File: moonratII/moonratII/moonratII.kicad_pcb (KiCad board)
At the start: 2 copper layers, 97.4 x 65.6 mm, 24 parts, among them J1 Barrel_Jack_Switch_SMT, J3 Conn_02x05_Odd_Even, J4 Screw_Terminal_01x06, J5 Screw_Terminal_01x06, J6 Conn_02x05_Odd_Even, J7 Screw_Terminal_01x02, Q1 IRF520N, Q2 BSS138, SW1 6mm 2 Pin Tact NO Breadboard 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, SW2 6mm 2 Pin Tact NO Breadboard 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, SW3 6mm 2 Pin Tact NO Breadboard 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, U1 TMP36xS

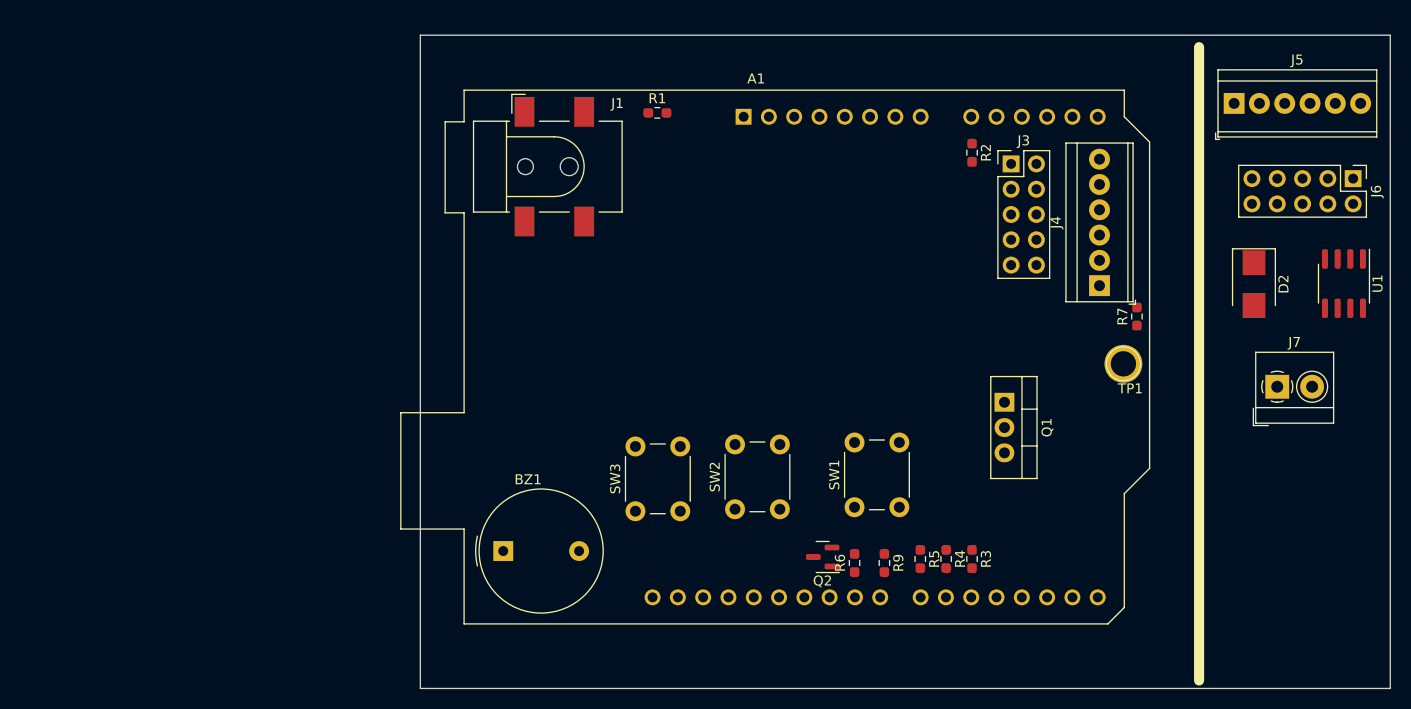
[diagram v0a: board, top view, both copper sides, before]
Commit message: Add more PCB 3D models. Place and lock down mounting holes.
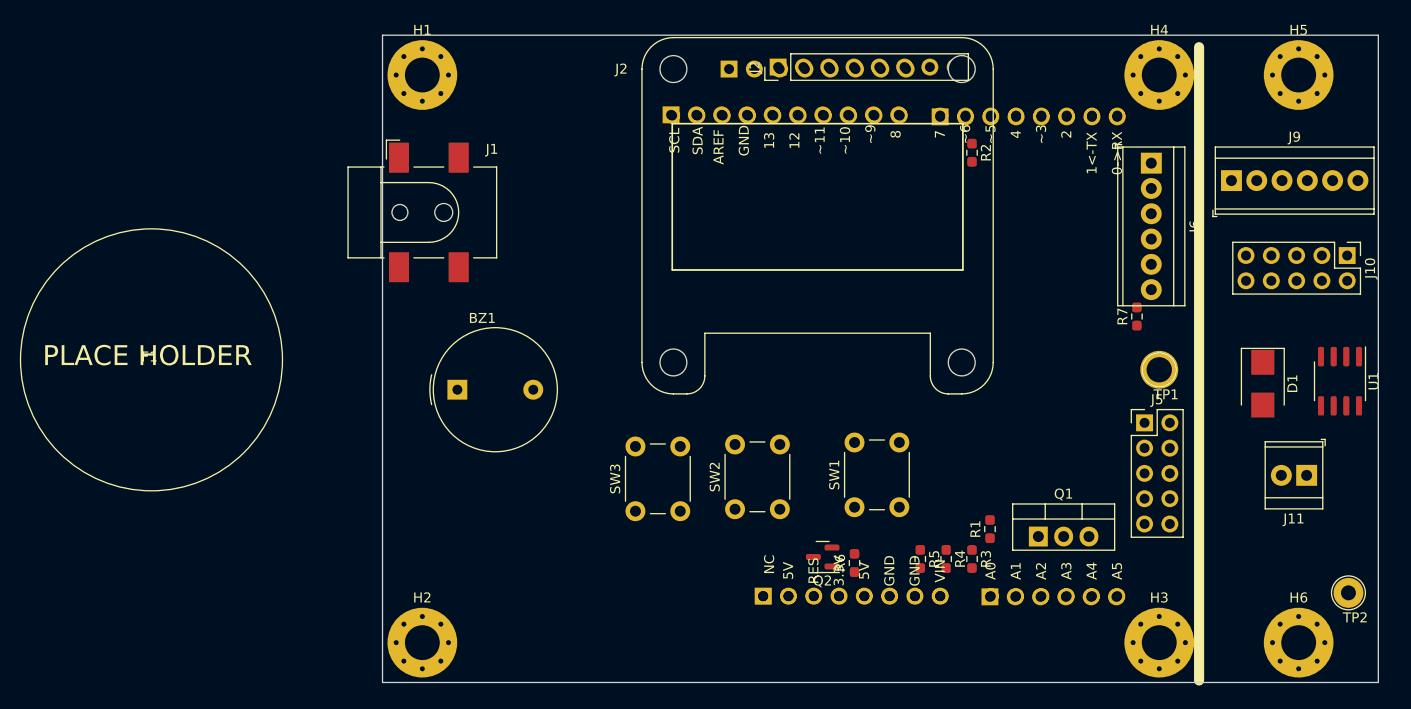
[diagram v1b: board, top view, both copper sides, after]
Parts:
- removed D2: Schottky 2A, Diode_SMD:D_SMB
- removed R9: 1K, Resistor_SMD:R_0603_1608Metric_Pad0.98x0.95mm_HandSolder
- added D1: Schottky 2A, Diode_SMD:D_SMB, F.Cu at (188.4, 95.0)
- added F1: Polyfuse 6A, GeneralPurposeAlarmDevicePCB:PlaceHolderOpossum, F.Cu at (76.6, 92.8)
- added H1: MountingHole_Pad_3.5mm, GeneralPurposeAlarmDevicePCB:MountingHole_3.5mm_Pad_Via, F.Cu at (104.0, 64.0)
- added H2: MountingHole_Pad_3.5mm, GeneralPurposeAlarmDevicePCB:MountingHole_3.5mm_Pad_Via, F.Cu at (104.0, 121.0)
- added H3: MountingHole_Pad_3.5mm, GeneralPurposeAlarmDevicePCB:MountingHole_3.5mm_Pad_Via, F.Cu at (178.0, 121.0)
- added H4: MountingHole_Pad_3.5mm, GeneralPurposeAlarmDevicePCB:MountingHole_3.5mm_Pad_Via, F.Cu at (178.0, 64.0)
- added H5: MountingHole_Pad_3.5mm, GeneralPurposeAlarmDevicePCB:MountingHole_3.5mm_Pad_Via, F.Cu at (192.0, 64.0)
- added H6: MountingHole_Pad_3.5mm, GeneralPurposeAlarmDevicePCB:MountingHole_3.5mm_Pad_Via, F.Cu at (192.0, 121.0)
- added J10: Conn_02x05_Odd_Even, Connector_PinHeader_2.54mm:PinHeader_2x05_P2.54mm_Vertical, F.Cu at (196.9, 82.1)
- added J11: Screw_Terminal_01x02, TerminalBlock_TE-Connectivity:TerminalBlock_TE_282834-2_1x02_P2.54mm_Horizontal, F.Cu at (192.8, 104.2)
- added J2: SSD1306 OLED, Display:Adafruit_SSD1306, F.Cu at (134.8, 63.4)
- added J2: SSD1306 OLED, Connector_PinHeader_2.54mm:PinHeader_1x08_P2.54mm_Vertical, F.Cu at (139.7, 63.2)
- added J8: PinHeader_1x10_P2.54mm_Vertical, Connector_PinHeader_2.54mm:PinHeader_1x10_P2.54mm_Vertical, B.Cu at (129.0, 68.0)
- added J9: Screw_Terminal_01x06, TerminalBlock_TE-Connectivity:TerminalBlock_TE_282834-6_1x06_P2.54mm_Horizontal, F.Cu at (185.2, 74.6)
- added TP2: TP_GND, TestPoint:TestPoint_Loop_D2.54mm_Drill1.5mm_Beaded, F.Cu at (197.0, 116.0)
- A1: footprint Module:Arduino_UNO_R3 -> GeneralPurposeAlarmDevicePCB:Arduino_UNO_R3_NoMountingHoles3D; moved to B.Cu
- J3: value Conn_02x05_Odd_Even -> PinHeader_1x06_P2.54mm_Vertical; footprint Connector_PinHeader_2.54mm:PinHeader_2x05_P2.54mm_Vertical -> Connector_PinHeader_2.54mm:PinHeader_1x06_P2.54mm_Vertical; moved to B.Cu
- J4: value Screw_Terminal_01x06 -> PinHeader_1x08_P2.54mm_Vertical; footprint TerminalBlock_TE-Connectivity:TerminalBlock_TE_282834-6_1x06_P2.54mm_Horizontal -> Connector_PinHeader_2.54mm:PinHeader_1x08_P2.54mm_Vertical; moved to B.Cu
- J5: value Screw_Terminal_01x06 -> Conn_02x05_Odd_Even; footprint TerminalBlock_TE-Connectivity:TerminalBlock_TE_282834-6_1x06_P2.54mm_Horizontal -> Connector_PinHeader_2.54mm:PinHeader_2x05_P2.54mm_Vertical
- J6: value Conn_02x05_Odd_Even -> Screw_Terminal_01x06; footprint Connector_PinHeader_2.54mm:PinHeader_2x05_P2.54mm_Vertical -> TerminalBlock_TE-Connectivity:TerminalBlock_TE_282834-6_1x06_P2.54mm_Horizontal
- J7: value Screw_Terminal_01x02 -> PinHeader_1x08_P2.54mm_Vertical; footprint TerminalBlock_4Ucon:TerminalBlock_4Ucon_1x02_P3.50mm_Horizontal -> Connector_PinHeader_2.54mm:PinHeader_1x08_P2.54mm_Vertical; moved to B.Cu
- R2: value 1R -> 1K
- moved R1 53.5 mm to (161.0, 109.6), turned to 90 degrees
- moved A1 48.2 mm to (138.2, 116.3)
- moved J4 46.0 mm to (138.2, 116.3), turned to -90 degrees
- moved J3 43.5 mm to (161.0, 116.4), turned to -90 degrees
- moved J7 43.4 mm to (156.0, 68.2), turned to -90 degrees
- moved J5 33.3 mm to (176.5, 98.9)
- moved J6 20.3 mm to (177.2, 72.8)
- moved BZ1 16.8 mm to (107.5, 95.6)
- moved Q1 13.9 mm to (165.9, 110.3), turned to 0 degrees
- moved J1 13.4 mm to (104.7, 77.8)
- moved U1 9.81 mm to (196.2, 94.8)
- moved TP1 3.65 mm to (178.0, 93.6)
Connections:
- J1 pad 1: Net-(J1-Pad1) -> Net-(F1-Pad2)
- J1 pad 4: Net-(J1-Pad1) -> Net-(F1-Pad2)
- J3 pad 1: HeaterDrive -> (no net)
- J3 pad 2: GND -> (no net)
- J3 pad 3: +5V -> (no net)
- J3 pad 4: TempOut -> (no net)
- J3 pad 5: VCC -> (no net)
- J3 pad 6: VCC -> (no net)
- J4 pad 1: GND -> (no net)
- J4 pad 2: VCC -> (no net)
- J4 pad 3: HeaterDrive -> (no net)
- J4 pad 4: +5V -> (no net)
- J4 pad 5: TempOut -> (no net)
- J4 pad 6: GND -> (no net)
- J5 pad 1: GND -> HeaterDrive
- J5 pad 2: VCC -> GND
- J5 pad 3: HeaterDrive -> +5V
- J5 pad 4: +5V -> TempOut
- J5 pad 5: TempOut -> VCC
- J5 pad 6: GND -> VCC
- J6 pad 1: HeaterDrive -> GND
- J6 pad 2: GND -> VCC
- J6 pad 3: +5V -> HeaterDrive
- J6 pad 4: TempOut -> +5V
- J6 pad 5: VCC -> TempOut
- J6 pad 6: VCC -> GND
- J7 pad 1: VCC -> (no net)
- J7 pad 2: Net-(D2-Pad2) -> (no net)
- R1 pad 1: Net-(J1-Pad1) -> TEMP_IN
- R1 pad 2: VCC -> TempOut
- R2 pad 1: TEMP_IN -> HEATER_ON
- R2 pad 2: TempOut -> Net-(A1-Pad23)
- SW1 pad 1: BTN_SELECT -> BTN_DOWN
- SW1 pad 2: BTN_SELECT -> BTN_DOWN
- SW2 pad 1: BTN_UP -> BTN_SELECT
- SW2 pad 2: BTN_UP -> BTN_SELECT
- SW3 pad 1: BTN_DOWN -> BTN_UP
- SW3 pad 2: BTN_DOWN -> BTN_UP
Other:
- board size 97.4 x 65.6 mm -> 100 x 65 mm
